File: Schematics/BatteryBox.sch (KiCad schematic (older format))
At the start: 1 part, among them P2 Conn_WallPlug

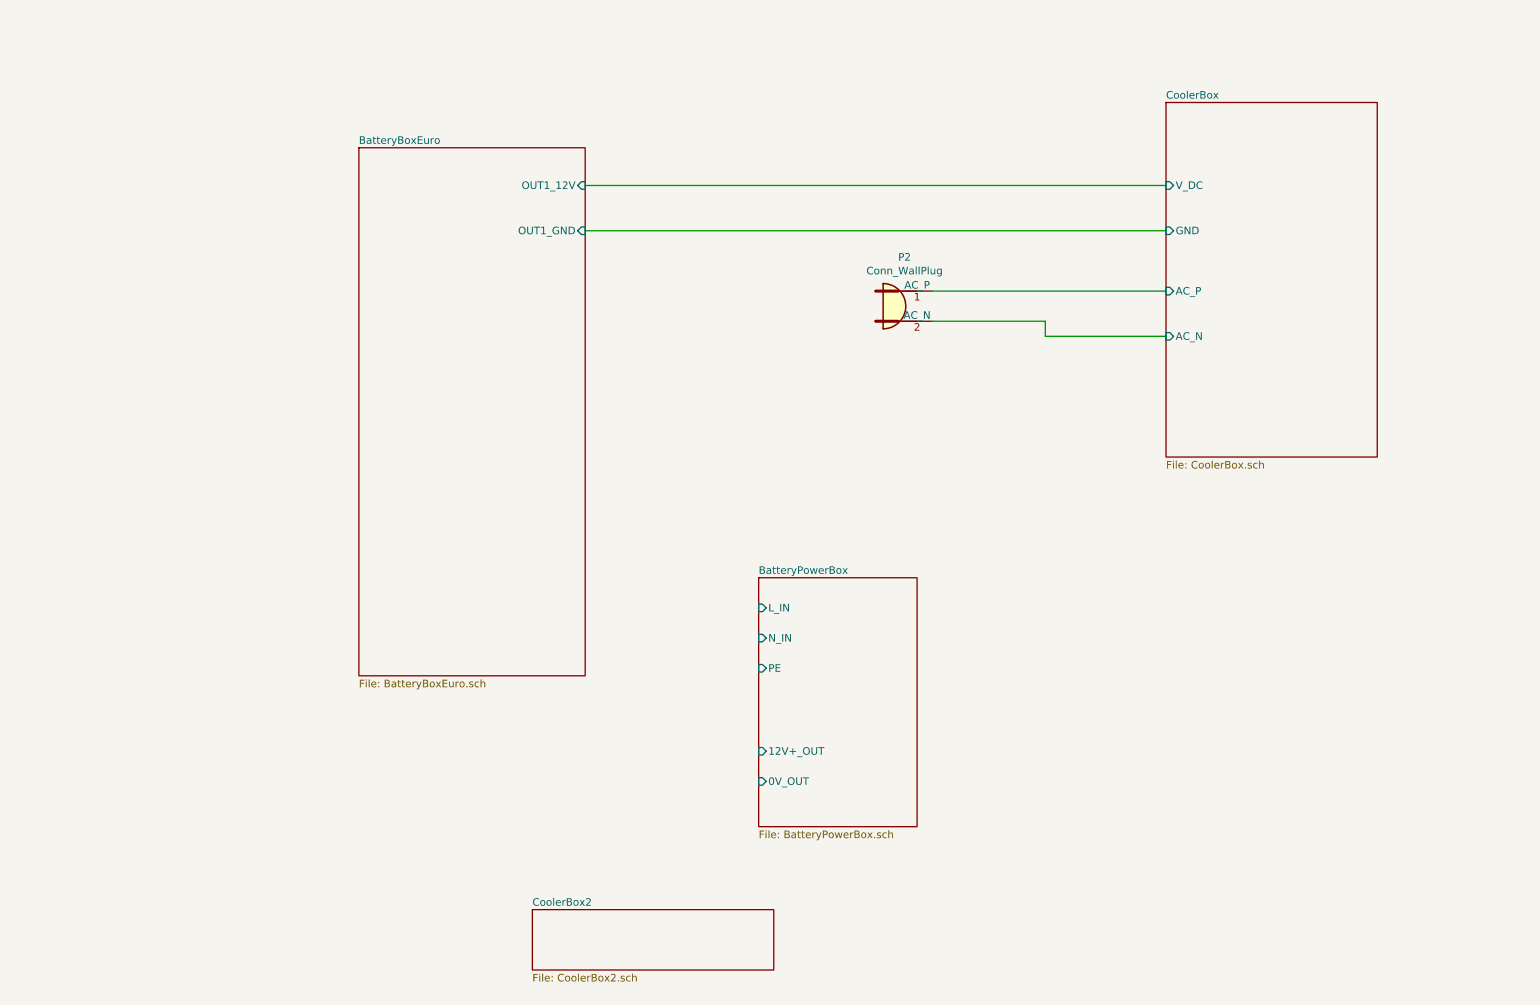
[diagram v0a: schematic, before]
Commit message: finalize schematic
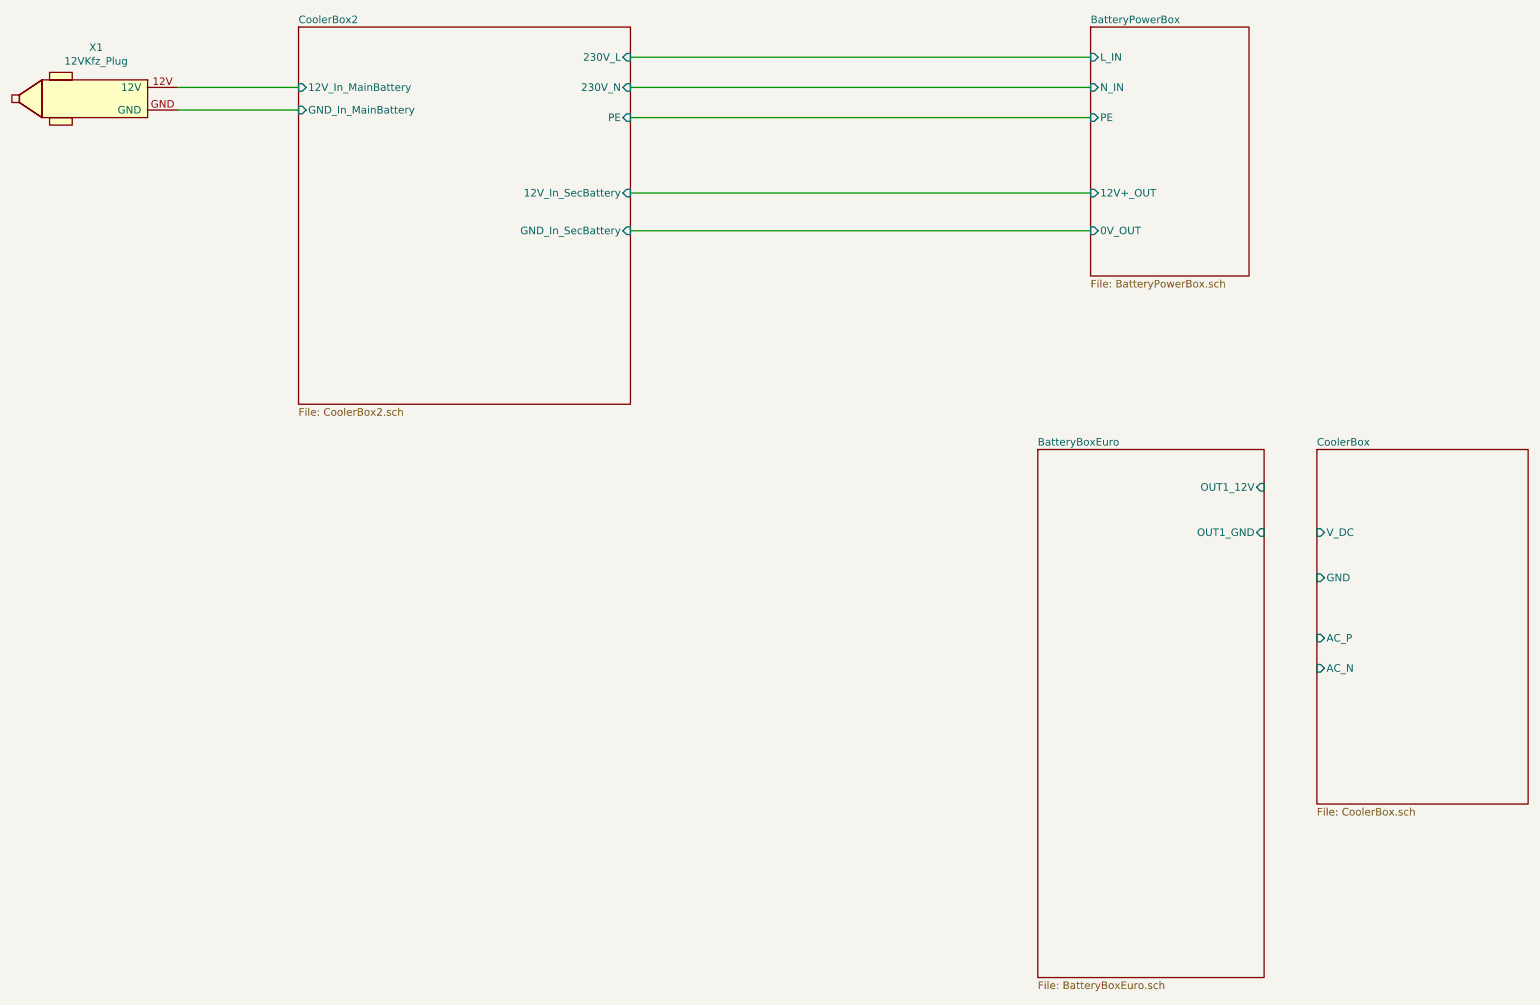
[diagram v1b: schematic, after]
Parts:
- removed P2: Conn_WallPlug, symbol Connector:Conn_WallPlug
- added X1: 12VKfz_Plug, symbol MyParts:12VKfz_Plug
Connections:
- new net CoolerBox2/12V_In_MainBattery: X1.12V
- new net CoolerBox2/GND_In_MainBattery: X1.GND
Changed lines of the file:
@@
 $EndDescr
 $Sheet
-S 8350 1450 1400 2350
+S 9350 3750 1400 2350
 U 5EF099A0
 F0 "CoolerBox" 50
 F1 "CoolerBox.sch" 50
-F2 "V_DC" I L 8350 2000 50
-F3 "GND" I L 8350 2300 50
-F4 "AC_P" I L 8350 2700 50
-F5 "AC_N" I L 8350 3000 50
+F2 "V_DC" I L 9350 4300 50
+F3 "GND" I L 9350 4600 50
+F4 "AC_P" I L 9350 5000 50
+F5 "AC_N" I L 9350 5200 50
 $EndSheet
 $Sheet
-S 3000 1750 1500 3500
+S 7500 3750 1500 3500
 U 5EF0A72F
 F0 "BatteryBoxEuro" 50
 F1 "BatteryBoxEuro.sch" 50
-F2 "OUT1_12V" I R 4500 2000 50
-F3 "OUT1_GND" I R 4500 2300 50
+F2 "OUT1_12V" I R 9000 4000 50
+F3 "OUT1_GND" I R 9000 4300 50
 $EndSheet
-Wire Wire Line
-	4500 2000 8350 2000
-Wire Wire Line
-	4500 2300 8350 2300
-$Comp
-L Connector:Conn_WallPlug P2
-U 1 1 5EF0BCF3
-P 6600 2800
-F 0 "P2" H 6617 3125 50  0000 C CNN
-F 1 "Conn_WallPlug" H 6617 3034 50  0000 C CNN
-F 2 "" H 7000 2800 50  0001 C CNN
-F 3 "~" H 7000 2800 50  0001 C CNN
-	1    6600 2800
-	1    0    0    -1
-$EndComp
-Wire Wire Line
-	6800 2700 8350 2700
-Wire Wire Line
-	6800 2900 7550 2900
-Wire Wire Line
-	7550 2900 7550 3000
-Wire Wire Line
-	7550 3000 8350 3000
 $Sheet
-S 5650 4600 1050 1650
+S 7850 950  1050 1650
 U 5F0C81D9
 F0 "BatteryPowerBox" 50
 F1 "BatteryPowerBox.sch" 50
-F2 "L_IN" I L 5650 4800 50
-F3 "N_IN" I L 5650 5000 50
-F4 "12V+_OUT" I L 5650 5750 50
-F5 "0V_OUT" I L 5650 5950 50
-F6 "PE" I L 5650 5200 50
+F2 "L_IN" I L 7850 1150 50
+F3 "N_IN" I L 7850 1350 50
+F4 "12V+_OUT" I L 7850 2050 50
+F5 "0V_OUT" I L 7850 2300 50
+F6 "PE" I L 7850 1550 50
 $EndSheet
+Wire Wire Line
+	4800 2300 7850 2300
 $Sheet
-S 4150 6800 1600 400
+S 2600 950  2200 2500
 U 5F0EC429
 F0 "CoolerBox2" 50
 F1 "CoolerBox2.sch" 50
+F2 "12V_In_MainBattery" I L 2600 1350 50
+F3 "GND_In_MainBattery" I L 2600 1500 50
+F4 "12V_In_SecBattery" I R 4800 2050 50
+F5 "GND_In_SecBattery" I R 4800 2300 50
+F6 "230V_L" I R 4800 1150 50
+F7 "230V_N" I R 4800 1350 50
+F8 "PE" I R 4800 1550 50
 $EndSheet
+Wire Wire Line
+	4800 2050 7850 2050
+Wire Wire Line
+	4800 1150 7850 1150
+Wire Wire Line
+	4800 1350 7850 1350
+Wire Wire Line
+	4800 1550 7850 1550
+$Comp
+L MyParts:12VKfz_Plug X1
+U 1 1 5F0D9E08
+P 1350 1200
+F 0 "X1" H 1442 1315 50  0000 C CNN
+F 1 "12VKfz_Plug" H 1442 1224 50  0000 C CNN
+F 2 "" H 1350 1200 50  0001 C CNN
+F 3 "" H 1350 1200 50  0001 C CNN
+	1    1350 1200
+	-1   0    0    -1
+$EndComp
+Wire Wire Line
+	1800 1350 2600 1350
+Wire Wire Line
+	1800 1500 2600 1500
 $EndSCHEMATC
